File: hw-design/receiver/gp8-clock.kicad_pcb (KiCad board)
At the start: 2 copper layers, 103.8 x 50.9 mm, 82 parts, among them P1 CONN_01X03, Q1 Q_NPN_BCE, Q2 Q_NPN_BCE, SW1 SW_PUSH, SW2 power, U1 TSOP39538, U2 weight-scale-lcd, U3 STM32F0-LQFP48, U4 usb-micro, U5 MCP73833, U6 AP1117D33, U7 nRF8001, Y1 Crystal, Y2 32kHz, Y3 16MHz

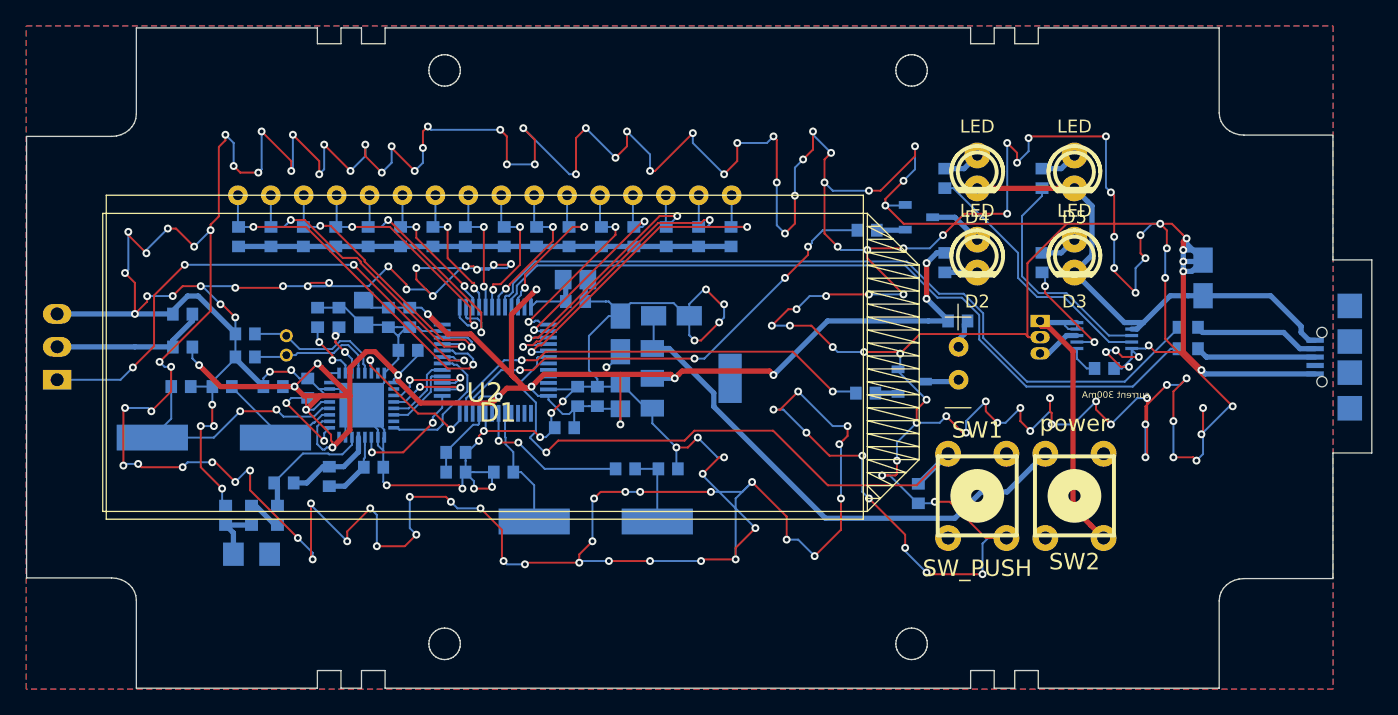
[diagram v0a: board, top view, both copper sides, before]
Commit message: Skończona rewizja r1, wysłane do satlanfd
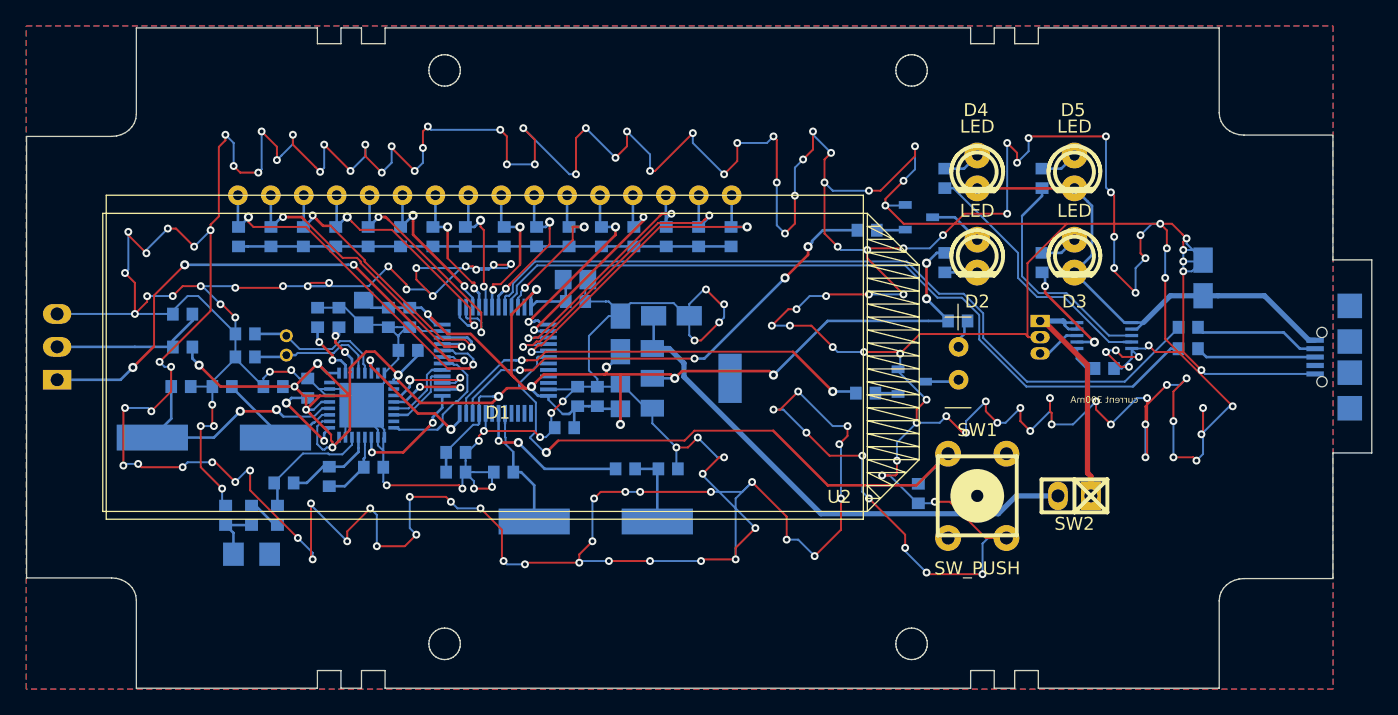
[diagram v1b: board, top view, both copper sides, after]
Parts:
- R25, R26, R27: value 560R -> 730R
- SW2: footprint w_switch:PCB_PUSH -> w_pin_strip:pin_socket_2
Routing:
- net Net-(P1-Pad1): track 24.1 -> 19.9 mm
- net GND: track 811.8 -> 809.8 mm
- net /seg2: track 11.7 -> 12.8 mm
- net /com1: track 28.3 -> 29.2 mm
- net /com3: track 22.3 -> 23.1 mm
- net Net-(C16-Pad1): track 41.0 -> 40.3 mm
- net /seg4: track 10.2 -> 10.8 mm
- net /com4: track 19.1 -> 19.7 mm
- net +5V: track 39.2 -> 39.8 mm
